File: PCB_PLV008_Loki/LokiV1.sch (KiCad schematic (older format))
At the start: 23 parts

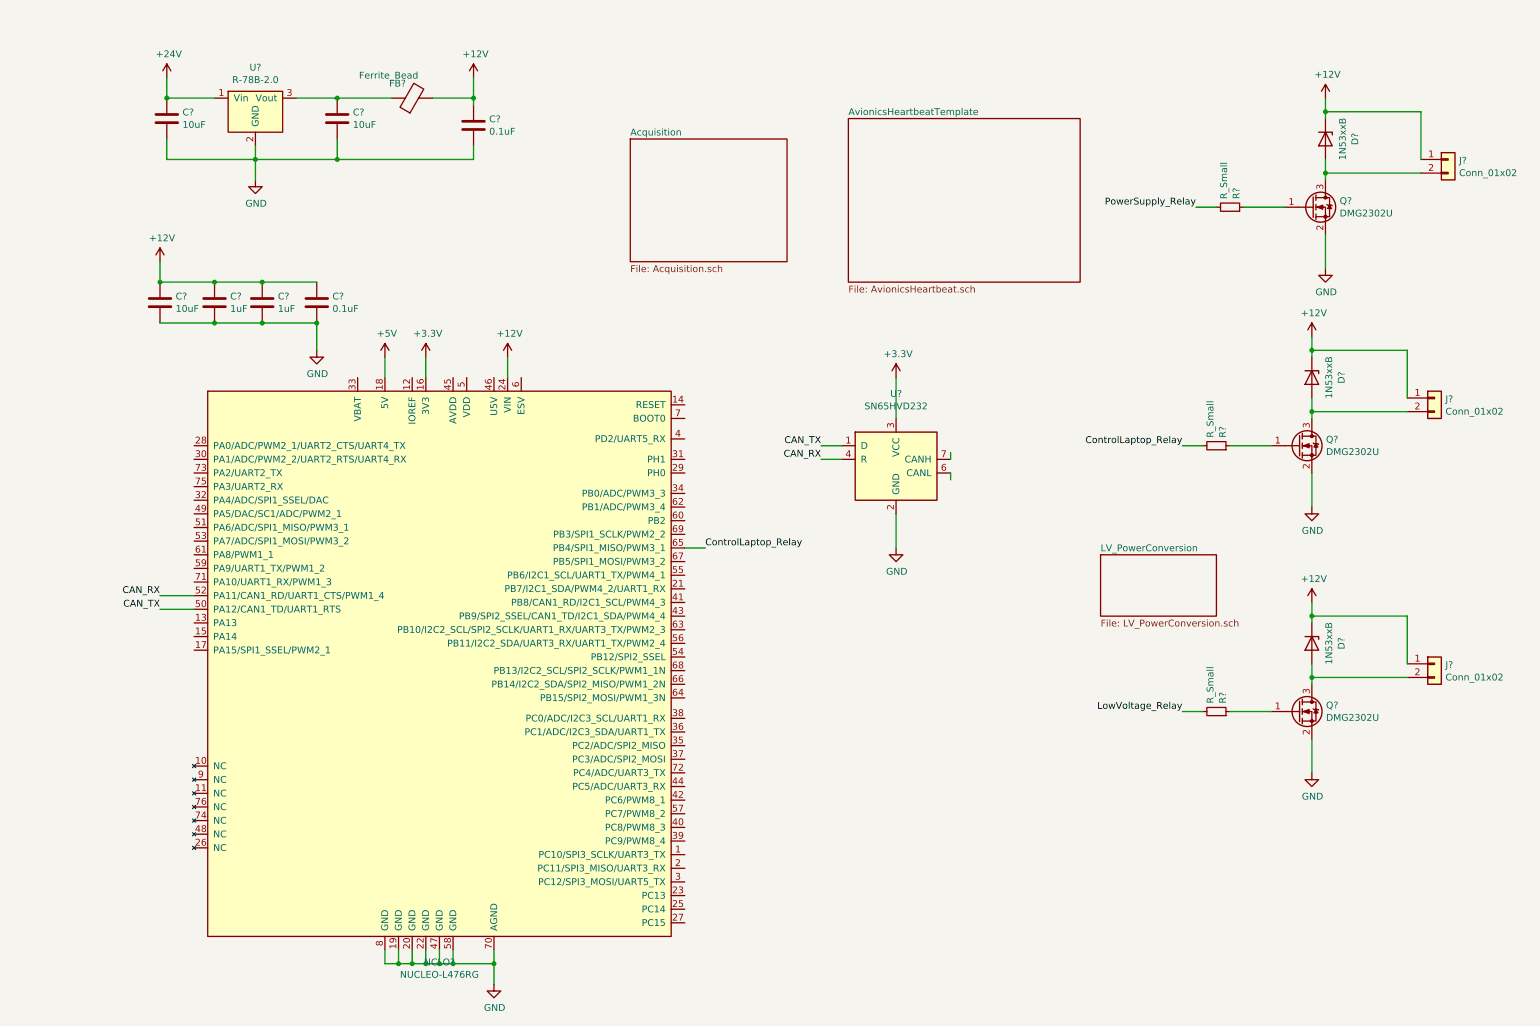
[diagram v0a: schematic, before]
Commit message: Add files via upload
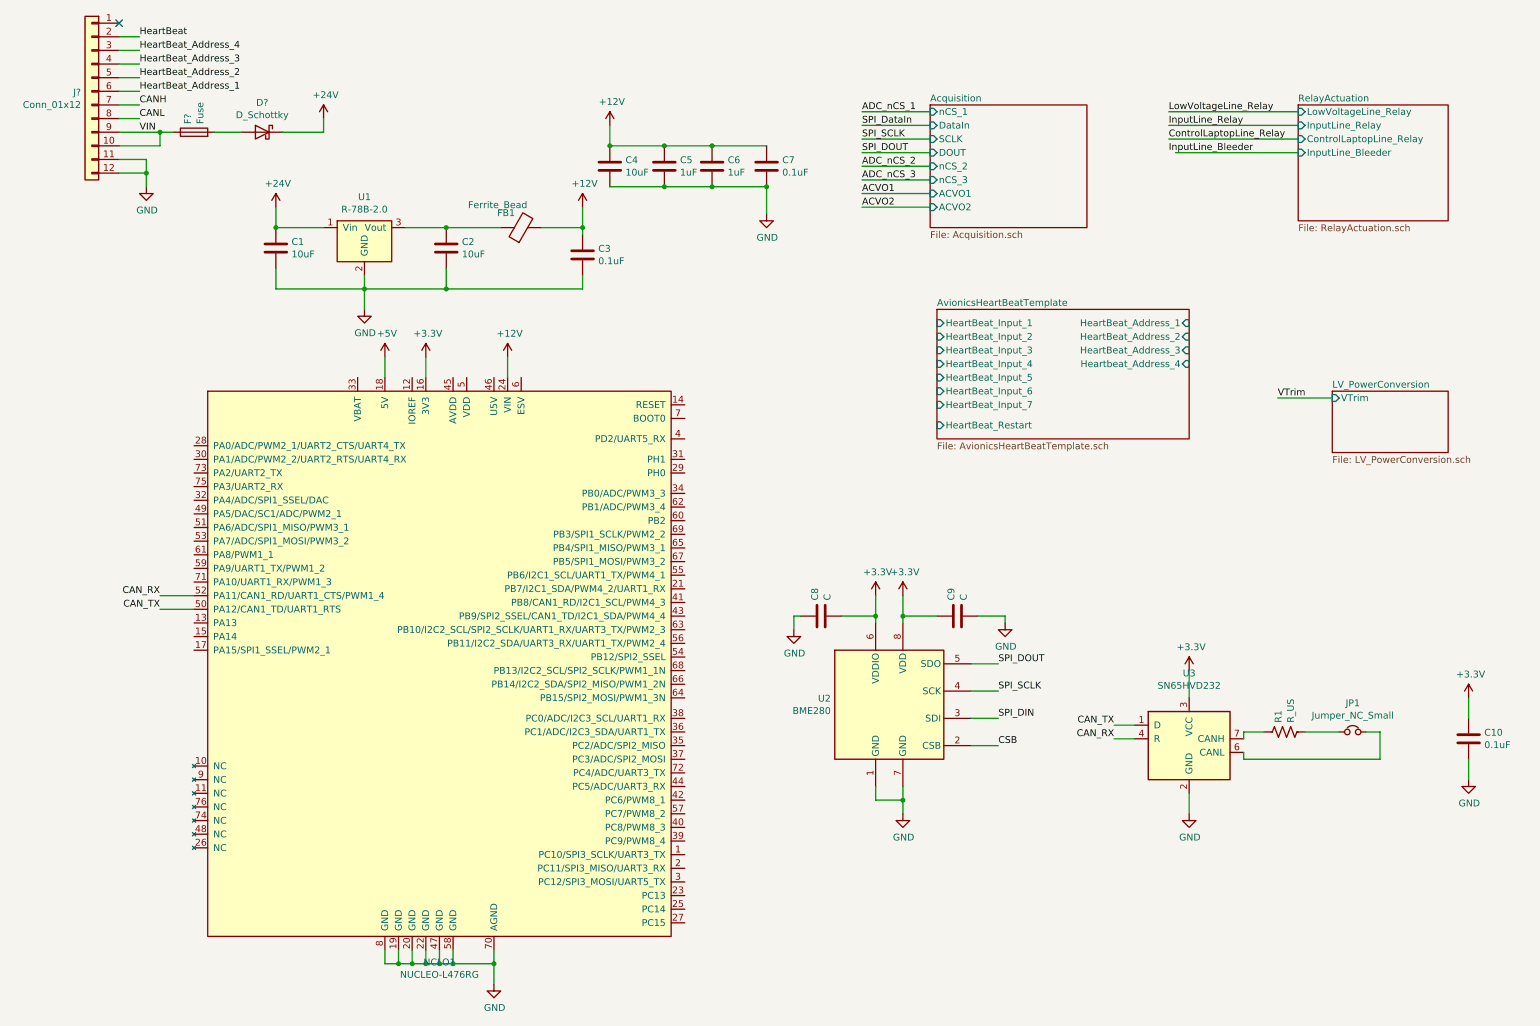
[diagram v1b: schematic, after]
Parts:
- removed D? (x3): 1N53xxB, Diode_THT:D_DO-201_P15.24mm_Horizontal, symbol Diode:1N53xxB
- removed J? (x3): Conn_01x02, symbol Connector_Generic:Conn_01x02
- removed Q? (x3): DMG2302U, Package_TO_SOT_SMD:SOT-23, symbol Transistor_FET:DMG2302U
- removed R? (x3): R_Small, symbol Device:R_Small
- added C10: 0.1uF, symbol Device:C
- added C8, C9: C, symbol Device:C
- added D?: D_Schottky, symbol Device:D_Schottky
- added F?: Fuse, symbol Device:Fuse
- added J?: Conn_01x12, symbol Connector_Generic:Conn_01x12
- added JP1: Jumper_NC_Small, symbol Device:Jumper_NC_Small
- added R1: R_US, symbol Device:R_US
- added U2: BME280, Package_LGA:Bosch_LGA-8_2.5x2.5mm_P0.65mm_ClockwisePinNumbering, symbol Sensor:BME280
- gave numbers to parts that had none: 11
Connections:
- net +24V: now also D?.1 (K)
- net +3V3: now also C10.1, C8.2, C9.1, U2.6 (VDDIO), U2.8 (VDD)
- net GND: now also C10.2, C8.1, C9.2, J?.11 (Pin_11), J?.12 (Pin_12), U2.1 (GND), U2.7 (GND)
- net at U3.6 (CANL): now also JP1.2
- net at U3.7 (CANH): now also R1.1
- net ControlLaptop_Relay: no longer names the net of NCLO1.65 (PB4/SPI1_MISO/PWM3_1)
- new net: JP1.1, R1.2
- new net: D?.2 (A), F?.2
- new net CANH: J?.7 (Pin_7)
- new net CANL: J?.8 (Pin_8)
- new net CSB: U2.2 (CSB)
- new net HeartBeat: J?.2 (Pin_2)
- new net HeartBeat_Address_1: J?.6 (Pin_6)
- new net HeartBeat_Address_2: J?.5 (Pin_5)
- new net HeartBeat_Address_3: J?.4 (Pin_4)
- new net HeartBeat_Address_4: J?.3 (Pin_3)
- new net SPI_DIN: U2.3 (SDI)
- new net SPI_DOUT: U2.5 (SDO)
- new net SPI_SCLK: U2.4 (SCK)
- new net VIN: F?.1, J?.10 (Pin_10), J?.9 (Pin_9)
- no-connect marks 0 -> 1
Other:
- moved on the sheet: C1, C2, C3, C4, C5, C6, C7, FB1, U1, U3
